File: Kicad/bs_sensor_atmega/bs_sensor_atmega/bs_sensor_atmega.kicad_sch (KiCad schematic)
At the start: 25 parts, among them J1 Conn_01x02, J2 Conn_01x04, J3 Conn_01x04, J4 Conn_01x04, U1 NRF24L01_Breakout, U2 AMS1117-3.3, U3 STM32F030F4Px, U4 ATmega48-20A, Y1 16MHz, Y2 16MHz

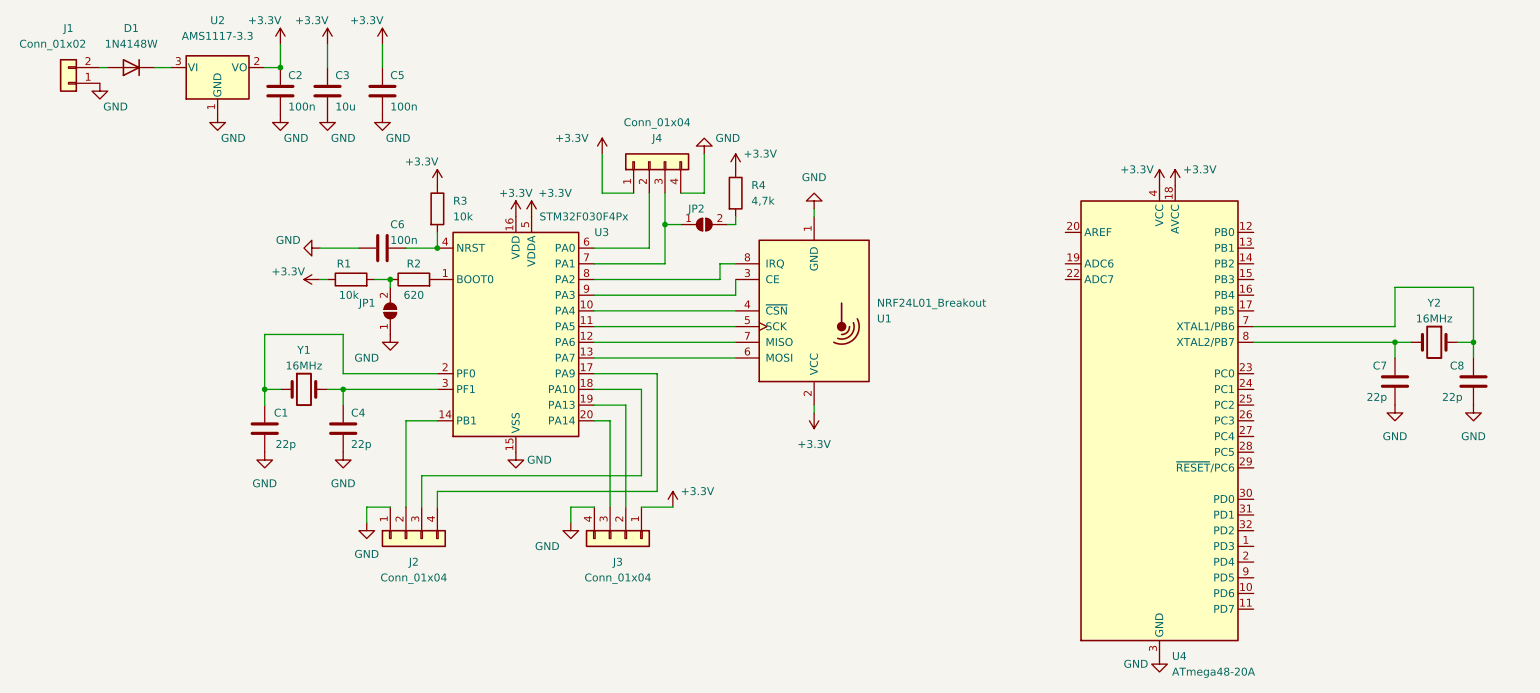
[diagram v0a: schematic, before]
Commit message: 07.03.2022
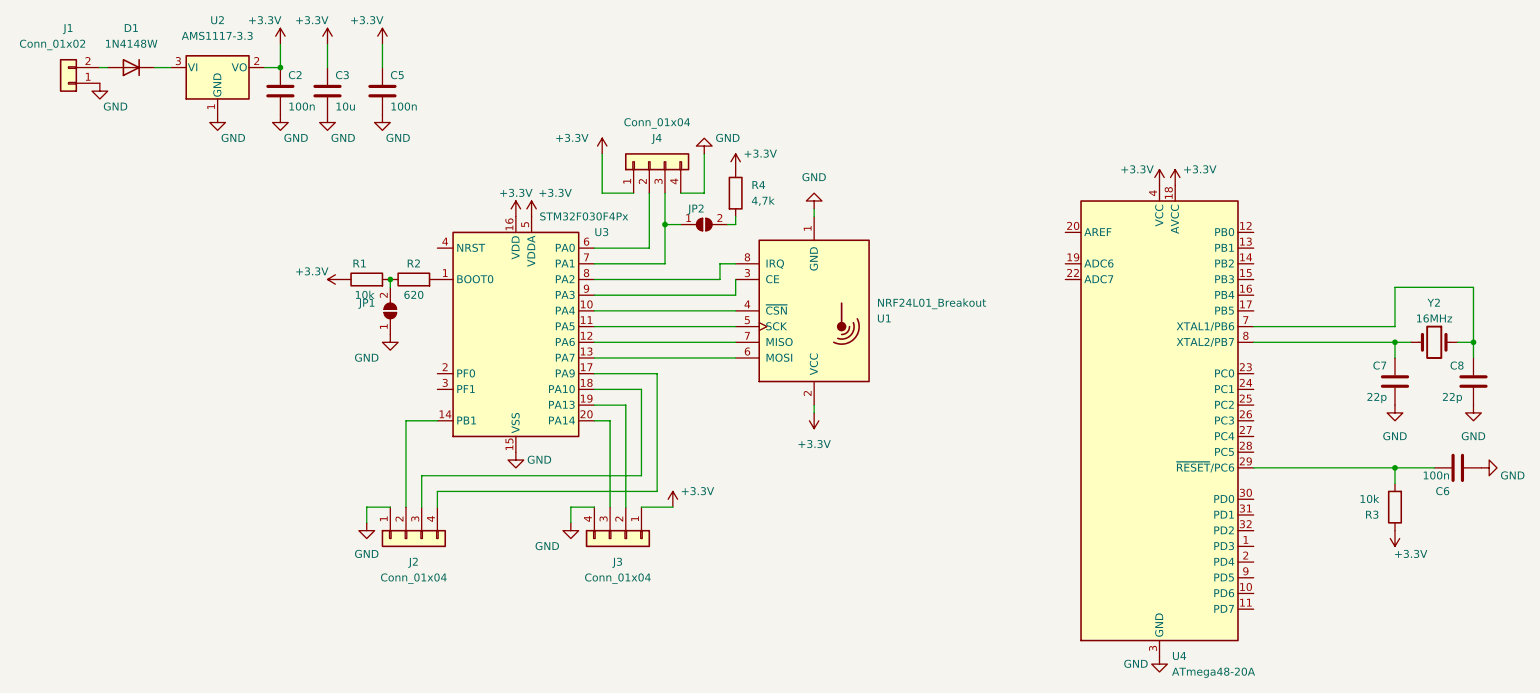
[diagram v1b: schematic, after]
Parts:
- removed C1, C4: 22p, Capacitor_SMD:C_0805_2012Metric, symbol Device:C
- removed Y1: 16MHz, Crystal:Crystal_HC49-U_Vertical, symbol Device:Crystal
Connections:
- net at U4.29 (~{RESET}/PC6): now also C6.1, R3.2
- now unconnected: U3.4 (NRST)
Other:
- moved on the sheet: C6, R1, R3
